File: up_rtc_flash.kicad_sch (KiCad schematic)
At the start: 1 part, among them J1 EduboardV2 PCIE UP Board Conn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

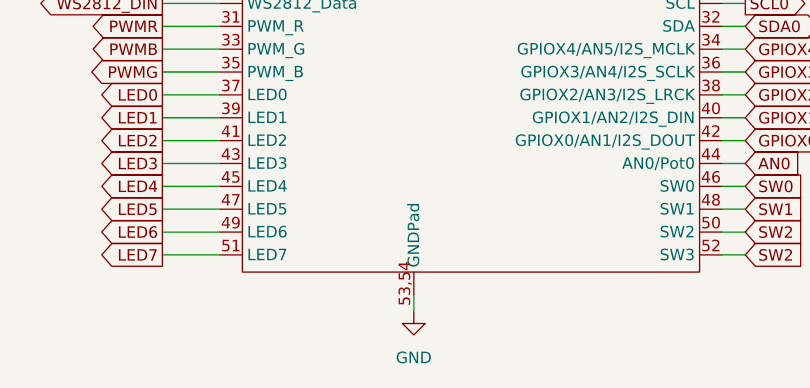
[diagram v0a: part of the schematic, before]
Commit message: Layout of parts done. Started laying tracks
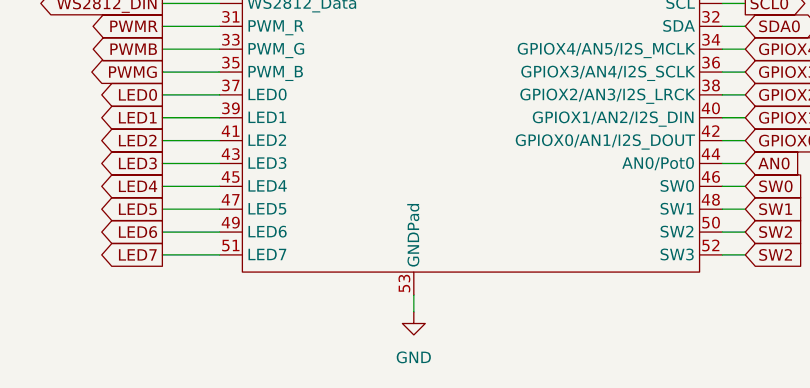
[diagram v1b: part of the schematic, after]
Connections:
- net GND: now also J1.53 (GNDPad), J1.54 (GNDPad); no longer J1.53,54 (GNDPad)
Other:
- moved on the sheet: J1
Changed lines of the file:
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@@
     (pin "51")
     (pin "52")
-    (pin "53,54")
+    (pin "53")
+    (pin "54")
     (pin "6")
     (pin "7")

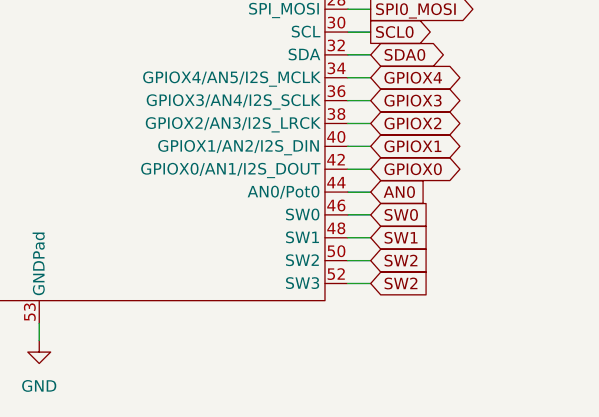
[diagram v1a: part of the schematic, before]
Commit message: proceed with layout
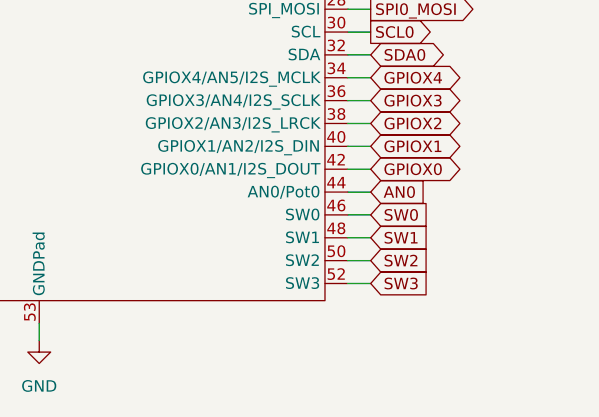
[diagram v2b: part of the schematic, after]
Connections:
- net SW2: no longer J1.52 (SW3)
- new net SW3: J1.52 (SW3)
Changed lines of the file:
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@@
     )
   )
-  (global_label "SW2" (shape input) (at 102.87 116.84 0) (fields_autoplaced)
+  (global_label "SW3" (shape input) (at 102.87 116.84 0) (fields_autoplaced)
     (effects (font (size 1.27 1.27)) (justify left))
-    (property "Intersheetrefs" "${INTERSHEET_REFS}" (at 109.1536 116.7606 0)
+    (property "Intersheetrefs" "${INTERSHEET_REFS}" (at 109.6462 116.84 0)
       (effects (font (size 1.27 1.27)) (justify left) hide)
     )
